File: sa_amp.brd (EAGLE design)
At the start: 160 x 50 mm, 96 parts, among them CN1 PCB Tab, CN2 PCB Tab, CN3 PCB Tab, CN4 PCB Tab, CN5 PCB Tab, CN6 PCB Tab, CN7 TC2030, CN8 NO FIT, Q1 2N7002, U1 STM32L031G6, U2 15V REG, U3 LM7812, U4 TPA3255, U5 LM317

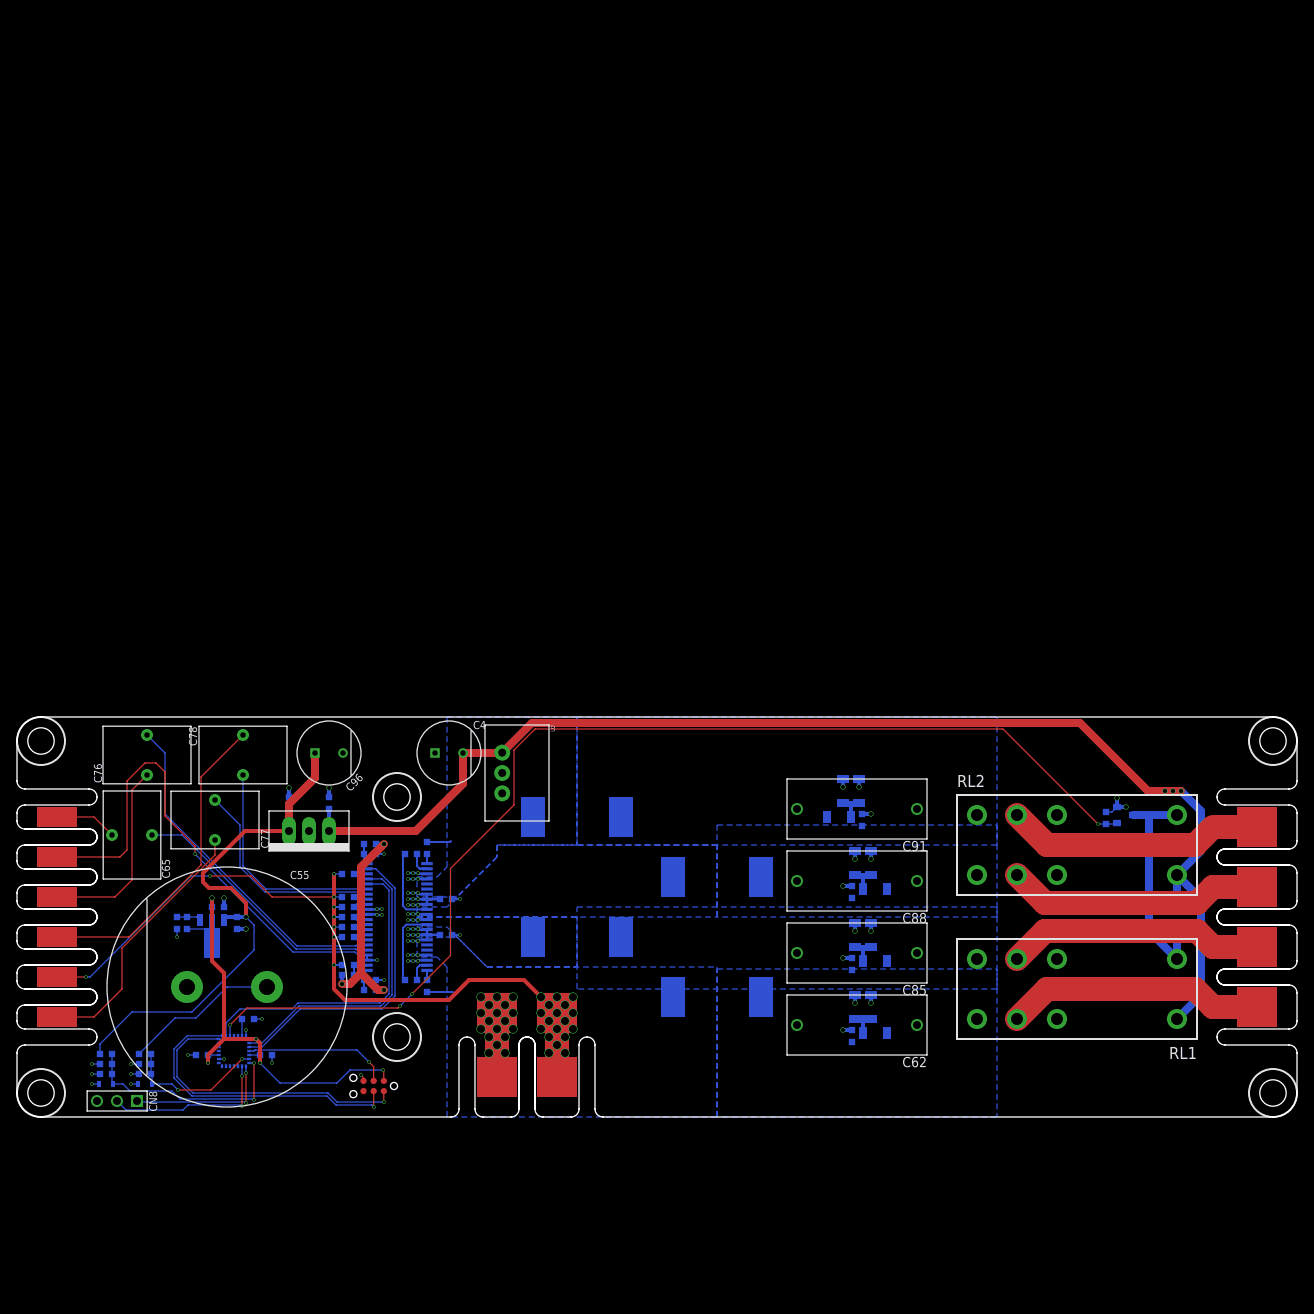
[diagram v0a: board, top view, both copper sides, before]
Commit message: amp fixed
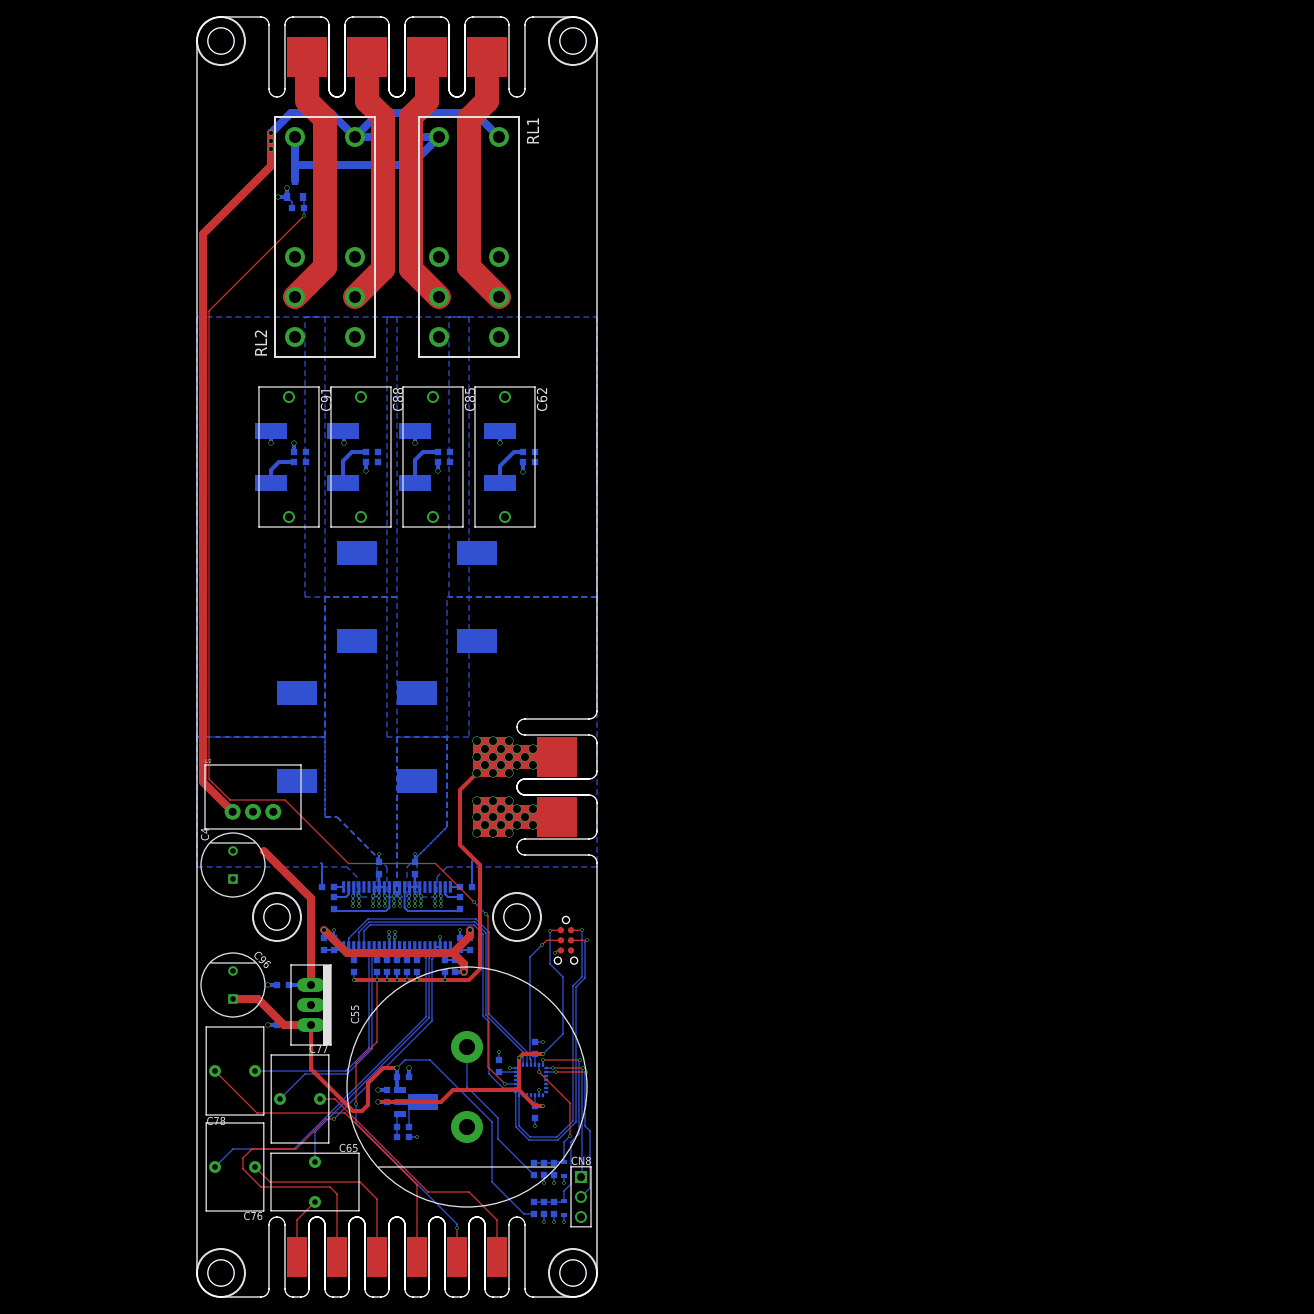
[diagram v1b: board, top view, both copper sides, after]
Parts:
- removed R33, R55, R57, R59: 2R0, RESISTORS:1206
- C63, C86, C89, C92: value 10nF 250V -> 1nF 50V
- C64, C87, C90, C93: value 220nF 100V -> 10nF 250V; device CAPACITORS:1206 -> CAPACITORS:0603
- R32, R54, R56, R58: value 2R0 -> 3R3; device RESISTORS:1206 -> RESISTORS:2512
- moved MECH3 158.0 mm to (22.0, 109.5), turned to 90 degrees
- moved MECH4 158.0 mm to (-22.0, 109.5), turned to 90 degrees
- moved HOLE1 152.9 mm to (11.2, 107.5), turned to 0 degrees
- moved HOLE4 152.9 mm to (-11.2, 107.5), turned to 0 degrees
- moved HOLE2 152.1 mm to (3.75, 107.5), turned to 0 degrees
- moved HOLE3 152.1 mm to (-3.75, 107.5), turned to 0 degrees
- moved D1 137.9 mm to (0.00, 97.5), turned to 0 degrees
- moved Q1 130.0 mm to (-12.8, 91.0), turned to 0 degrees
- moved R1 126.6 mm to (-12.4, 88.6), turned to 180 degrees
- moved RL1 120.9 mm to (9.00, 85.0), turned to 270 degrees
- moved RL2 120.9 mm to (-9.00, 85.0), turned to 270 degrees
- moved C64 84.5 mm to (16.5, 58.1), turned to 180 degrees
- moved C92 84.0 mm to (-12.1, 58.1), turned to 180 degrees
- moved C62 83.5 mm to (13.5, 57.5), turned to 270 degrees
- moved C91 83.5 mm to (-13.5, 57.5), turned to 270 degrees
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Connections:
- net 15V: now also C4.P; no longer C4.N
- net GND: now also C4.N; no longer C4.P, R33.1, R55.1, R57.1, R59.1
- net N$60: no longer R33.2
- net N$87: no longer R55.2
- net N$88: no longer R57.2
- net N$89: no longer R59.2
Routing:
- net 15V: track 159.9 -> 151.2 mm
- net N$87: track 3.75 -> 6.16 mm
- net N$88: track 3.75 -> 6.09 mm
- net N$60: track 3.75 -> 5.72 mm
- net GND: track 263.1 -> 261.5 mm, vias 86 -> 82
- net N$89: track 3.75 -> 4.91 mm
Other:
- board size 160 x 50 mm -> 50 x 160 mm
